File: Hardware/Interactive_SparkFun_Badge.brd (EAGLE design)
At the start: 68.5 x 102.6 mm, 31 parts, among them J1 AVR_SPI_PRG_6NS, U1 ATMEGA328P, Y1 8MHZ

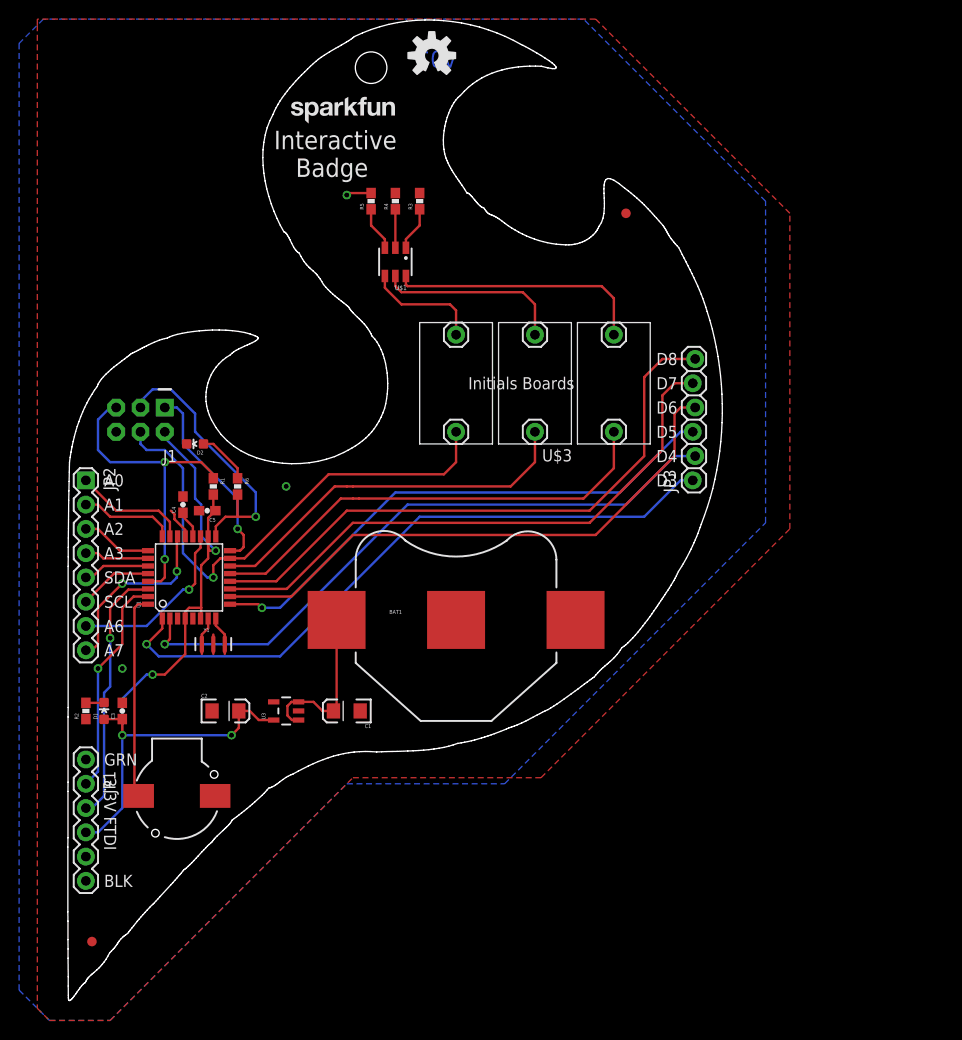
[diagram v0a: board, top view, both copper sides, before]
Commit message: New board design
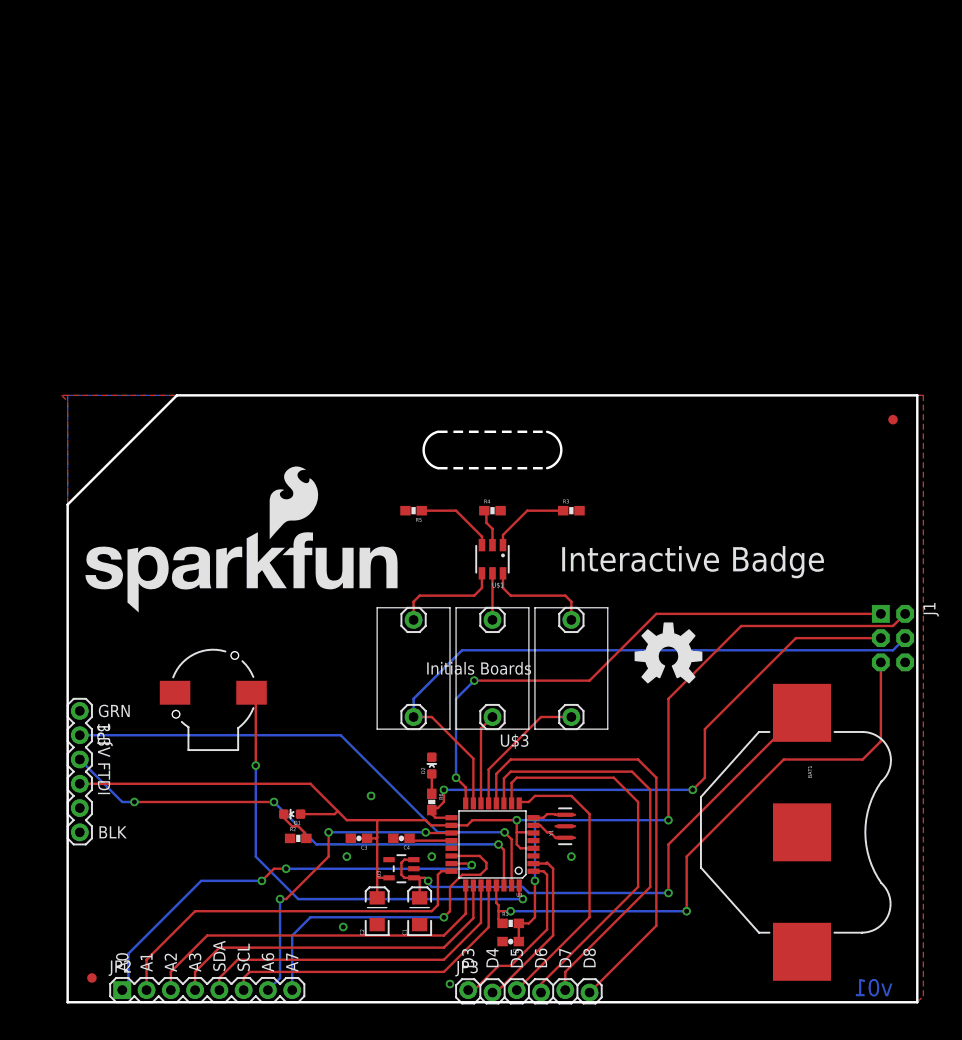
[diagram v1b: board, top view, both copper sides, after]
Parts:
- removed STANDOFF1: STAND-OFF, SparkFun-Electromechanical:STAND-OFF
- removed U$2: FLAME, Local Library:FLAME
- LOGO1: value OSHW-LOGOM -> OSHW-LOGOL; device SparkFun-Aesthetics:OSHW-LOGO-M -> SparkFun-Aesthetics:OSHW-LOGO-L
- LOGO2: value SFE_LOGO_NAME.1_INCH -> SFE_LOGO_NAME_FLAME.3_INCH; device SparkFun-Aesthetics:SFE_LOGO_NAME_.1 -> SparkFun-Aesthetics:SFE_LOGO_NAME_FLAME_.3
- moved J1 82.0 mm to (86.4, 38.1), turned to 270 degrees
- moved LOGO1 67.6 mm to (62.9, 36.2)
- moved JP3 58.3 mm to (41.9, 1.27), turned to 0 degrees
- moved R1 55.3 mm to (46.4, 8.26), turned to 0 degrees
- moved LOGO2 55.2 mm to (1.27, 40.6)
- moved C5 55.1 mm to (46.4, 6.35)
- moved JP2 53.5 mm to (5.71, 1.27), turned to 0 degrees
- moved BAT1 42.5 mm to (76.8, 17.8), turned to 270 degrees
- moved U1 42.3 mm to (44.5, 16.5), turned to 180 degrees
- moved D2 41.8 mm to (38.1, 24.8), turned to 0 degrees
- moved C4 41.7 mm to (34.9, 17.1), turned to 180 degrees
- moved Y1 41.5 mm to (52.1, 18.4), turned to 90 degrees
- moved R6 38.8 mm to (38.1, 21.0)
- moved R3 36.1 mm to (52.7, 51.4), turned to 0 degrees
- moved FID2 35.3 mm to (86.4, 61.0)
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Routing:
- net VCC: track 84.2 -> 139.5 mm, vias 4 -> 3
- net D3: track 68.7 -> 18.2 mm, vias 1 -> 0
- net D4: track 66.6 -> 18.2 mm, vias 1 -> 0
- net RAW: track 17.4 -> 58.8 mm, vias 0 -> 2
- net MISO: track 20.3 -> 59.5 mm, vias 1 -> 2
- net D9: track 48.5 -> 14.5 mm
- net A0: track 12.1 -> 46.1 mm, vias 0 -> 3
- net SCK: track 29.3 -> 60.8 mm, vias 1 -> 2
- net TXO: track 23.2 -> 54.5 mm
- net A1: track 9.99 -> 40.8 mm
- net A2: track 7.45 -> 38.2 mm
- net RESET: track 33.1 -> 63.2 mm
- net A3: track 6.73 -> 36.8 mm
- net D10: track 39.6 -> 9.54 mm
- net SDA: track 7.00 -> 34.9 mm
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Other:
- board size 68.5 x 102.6 mm -> 88.9 x 63.5 mm
